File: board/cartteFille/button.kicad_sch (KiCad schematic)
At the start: 13 parts, among them U21-2 SN74LVC2G14DBVTG4

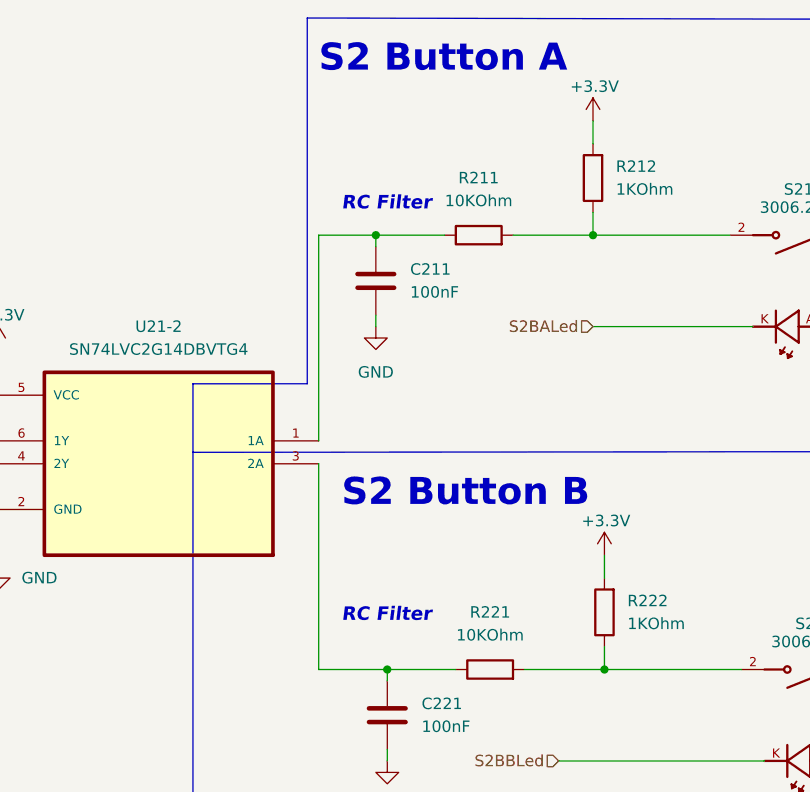
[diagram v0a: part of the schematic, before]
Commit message: litle change
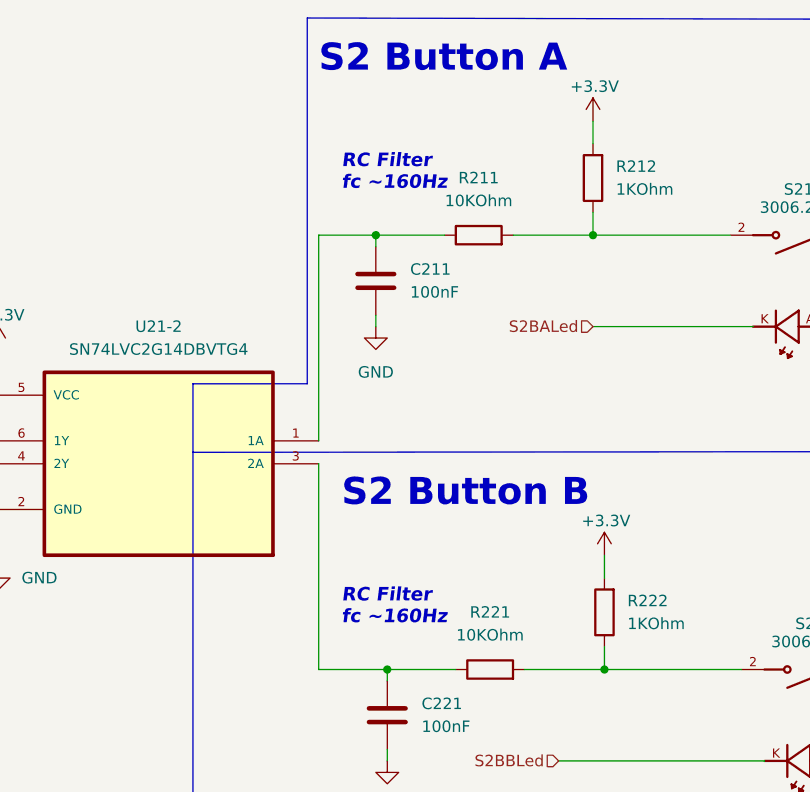
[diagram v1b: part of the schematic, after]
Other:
- note added: "RC Filter fc ~160Hz"
- note removed: "RC Filter"
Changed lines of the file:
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@@
     (effects (font (size 1.5 1.5)) (justify left bottom))
+  )
+  (text "RC Filter\nfc ~160Hz" (at 77.47 69.85 0)
+    (effects (font (size 1.5 1.5) (thickness 0.3) bold italic) (justify left bottom))
   )
   (text "2.1" (at 236.22 117.475 0)
@@
     (effects (font (size 1.5 1.5) (thickness 1) bold) (justify left bottom))
   )
-  (text "RC Filter" (at 77.47 117.856 0)
-    (effects (font (size 1.5 1.5) (thickness 0.3) bold italic) (justify left bottom))
-  )
   (text "3.3k" (at 255.27 95.885 0)
     (effects (font (size 1.5 1.5)) (justify left bottom))
@@
   (text "2.1" (at 236.22 90.805 0)
     (effects (font (size 1.5 1.5)) (justify left bottom))
+  )
+  (text "RC Filter\nfc ~160Hz" (at 77.47 118.11 0)
+    (effects (font (size 1.5 1.5) (thickness 0.3) bold italic) (justify left bottom))
   )
   (text "150" (at 255.27 90.805 0)
@@
     (effects (font (size 1.5 1.5)) (justify left bottom))
   )
-  (text "RC Filter" (at 77.47 72.136 0)
-    (effects (font (size 1.5 1.5) (thickness 0.3) bold italic) (justify left bottom))
-  )
   (text "3.3" (at 209.55 117.475 0)
